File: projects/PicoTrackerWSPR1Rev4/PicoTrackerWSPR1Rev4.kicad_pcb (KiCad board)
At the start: 2 copper layers, 69.5 x 24.8 mm, 54 parts, among them J1 Conn_01x02, M1 SIP32431DR3-T1GE3, M2 SIP32431DR3-T1GE3, M3 UBLOX_NEO-6, M4 SI5351A, U1 ATMEGA328P-AU, Y1 CRYSTAL_ABM8G

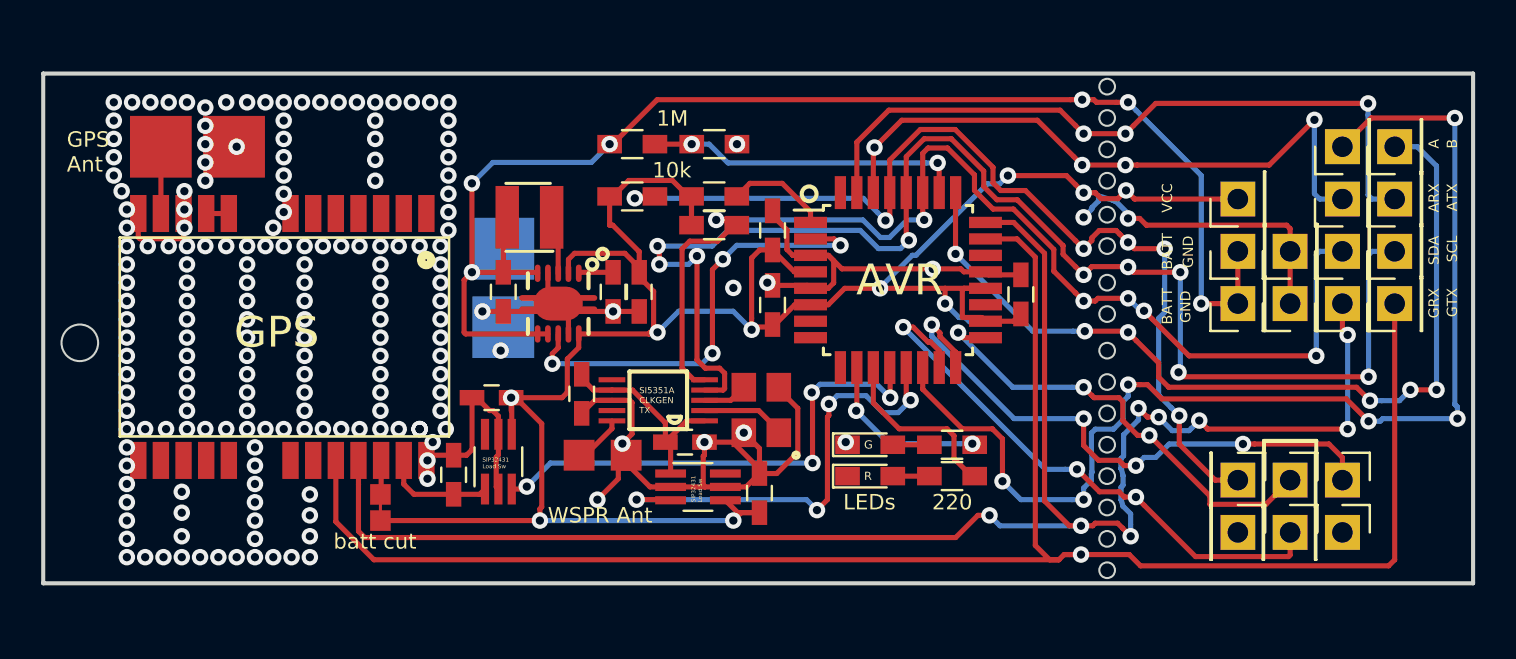
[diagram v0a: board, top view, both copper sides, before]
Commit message: KiCad PicoTrackerWSPR1Rev4 done
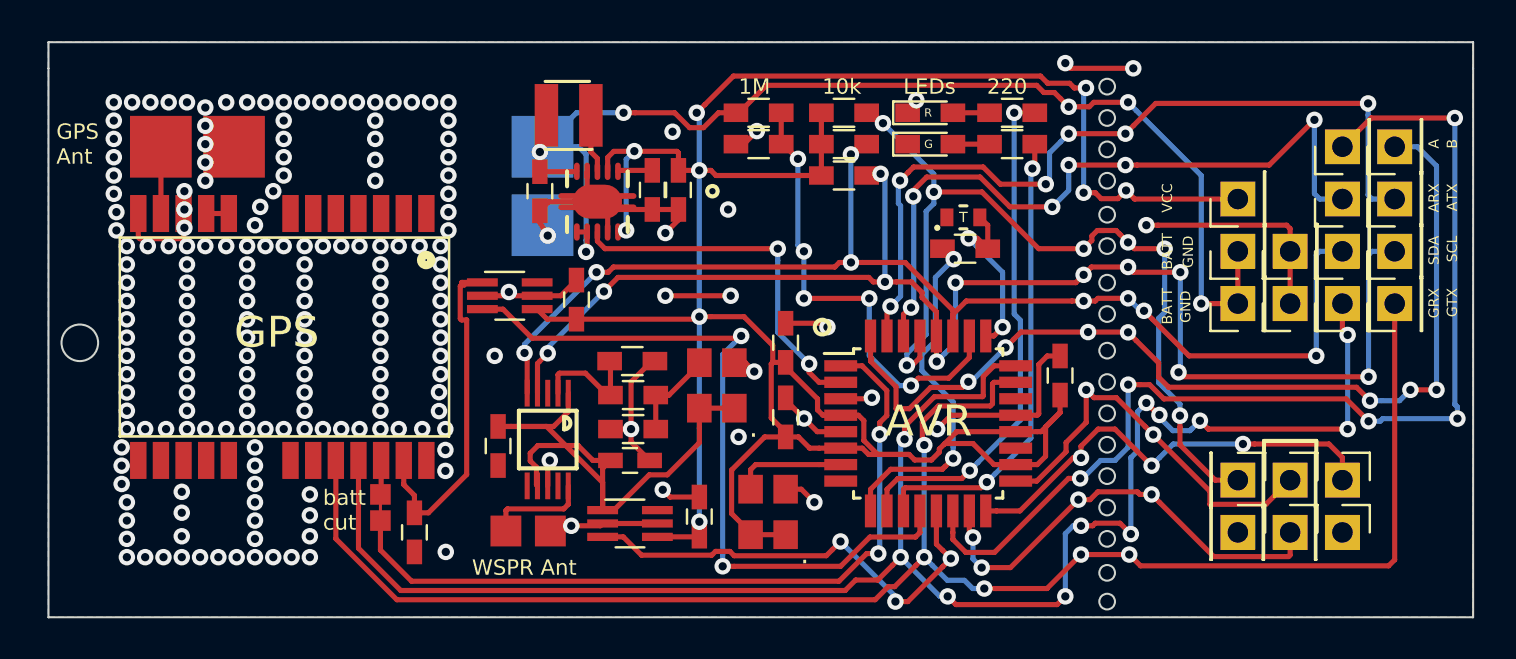
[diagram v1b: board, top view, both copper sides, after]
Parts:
- removed Y1: CRYSTAL_ABM8G, CustomFootprintLibrary:ABM8G-25.000MHZ-B4Y-T
- added R10: 68, Resistors_SMD:R_0603_HandSoldering, F.Cu at (82.4, 79.4)
- added R11: 100, Resistors_SMD:R_0603_HandSoldering, F.Cu at (82.3, 77.7)
- added R5: R_Small, Resistors_SMD:R_0603_HandSoldering, F.Cu at (98.5, 72.3)
- added R9: 100, Resistors_SMD:R_0603_HandSoldering, F.Cu at (82.4, 81.0)
- added TCXO1: CRYSTAL_TCXO_3.2mmWidth_2.5mmHeight, CustomFootprintLibrary:CRYSTAL_3.2mmWidth_2.5mmHeight, F.Cu at (88.9, 85.1)
- added TCXO2: CRYSTAL_TCXO_3.2mmWidth_2.5mmHeight, CustomFootprintLibrary:CRYSTAL_3.2mmWidth_2.5mmHeight, F.Cu at (86.4, 78.9)
- added TH1: PT100, CustomFootprintLibrary:PTS060301B100RP100, F.Cu at (98.4, 70.7)
- moved R1 16.4 mm to (100.8, 65.7)
- moved R2 16.4 mm to (100.8, 67.2)
- moved D1 16.4 mm to (96.8, 65.7)
- moved D2 16.4 mm to (96.8, 67.2)
- moved R6 10.3 mm to (92.6, 68.7)
- moved M1 8.08 mm to (76.4, 74.5), turned to 0 degrees
- moved R3 7.50 mm to (92.6, 65.7)
- moved R4 7.44 mm to (92.6, 67.2)
- moved U1 7.12 mm to (96.7, 80.8)
- moved R7 6.32 mm to (88.5, 65.7)
- moved C6 6.30 mm to (79.6, 74.7), turned to 270 degrees
- moved M4 5.70 mm to (78.2, 81.5), turned to 90 degrees
- moved C11 5.50 mm to (89.8, 80.5)
- moved C9 5.50 mm to (89.8, 76.8)
- moved C3 5.31 mm to (83.3, 69.4)
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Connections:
- J1 pad 1: VCC -> GPS_V_BCKP
- M4 pad 3: Net-(M4-Pad3) -> (no net)
- R3 pad 2: RESET -> SPI_RESET
- R6 pad 2: SPI_RESET -> SCL
- U1 pad 1: RESET -> GPS_V_BCKP
- U1 pad 25: SIG_B -> VTEMP_SENSE
- U1 pad 32: (no net) -> SIG_B
- U1 pad 7: (no net) -> Net-(TCXO1-Pad3)
- U1 pad 9: (no net) -> TEMP_ENABLE
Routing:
- net GPS_V_BCKP: track 0.00 -> 37.5 mm, vias 0 -> 2
- net VCC: track 110.3 -> 134.0 mm, vias 10 -> 9
- net WSPR_VCC: track 10.1 -> 30.3 mm
- net TEMP_ENABLE: track 0.00 -> 17.4 mm, vias 0 -> 2
- net LED_1: track 8.55 -> 25.0 mm
- net GND: track 91.5 -> 75.2 mm, vias 187 -> 195
- net LED_2: track 8.77 -> 22.6 mm, vias 0 -> 2
- net GPS_ENABLE: track 24.3 -> 36.1 mm, vias 4 -> 2
- net GPS_VCC: track 5.41 -> 16.9 mm
- net VBATT: track 68.6 -> 59.5 mm
- net VTEMP_SENSE: track 0.00 -> 8.82 mm, vias 0 -> 2
- net VBATT_SENSE: track 15.6 -> 22.6 mm, vias 2 -> 5
- net SPI_MISO: track 28.3 -> 21.8 mm, vias 4 -> 3
- net SPI_MOSI: track 27.6 -> 21.9 mm, vias 3 -> 4
- net Net-(TCXO1-Pad3): track 0.00 -> 5.43 mm
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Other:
- board size 69.5 x 24.8 mm -> 69.2 x 27.9 mm
- board text added: "2019-05-01 PicoTrackerWSPR1 Rev 4"
- board text removed: "2019-03-27 PicoTrackerWSPR1 Rev 3"
- board text removed: "SI5351A CLKGEN TX"
- board text removed: "SIP32431 Load Sw"
